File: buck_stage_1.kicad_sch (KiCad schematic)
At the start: 30 parts

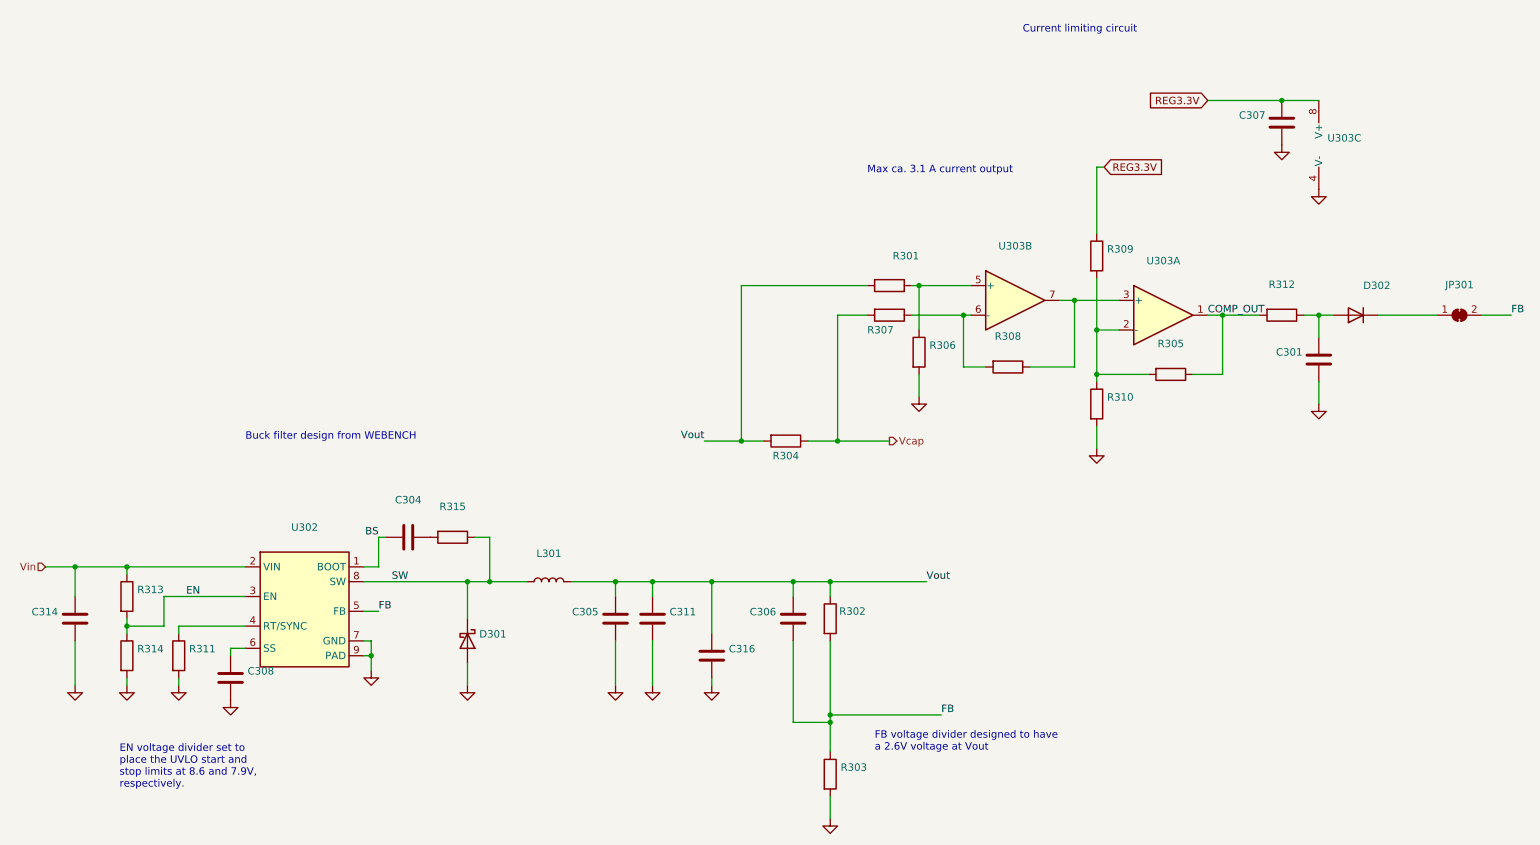
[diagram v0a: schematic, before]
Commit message: SH-RPi v2 schematic design
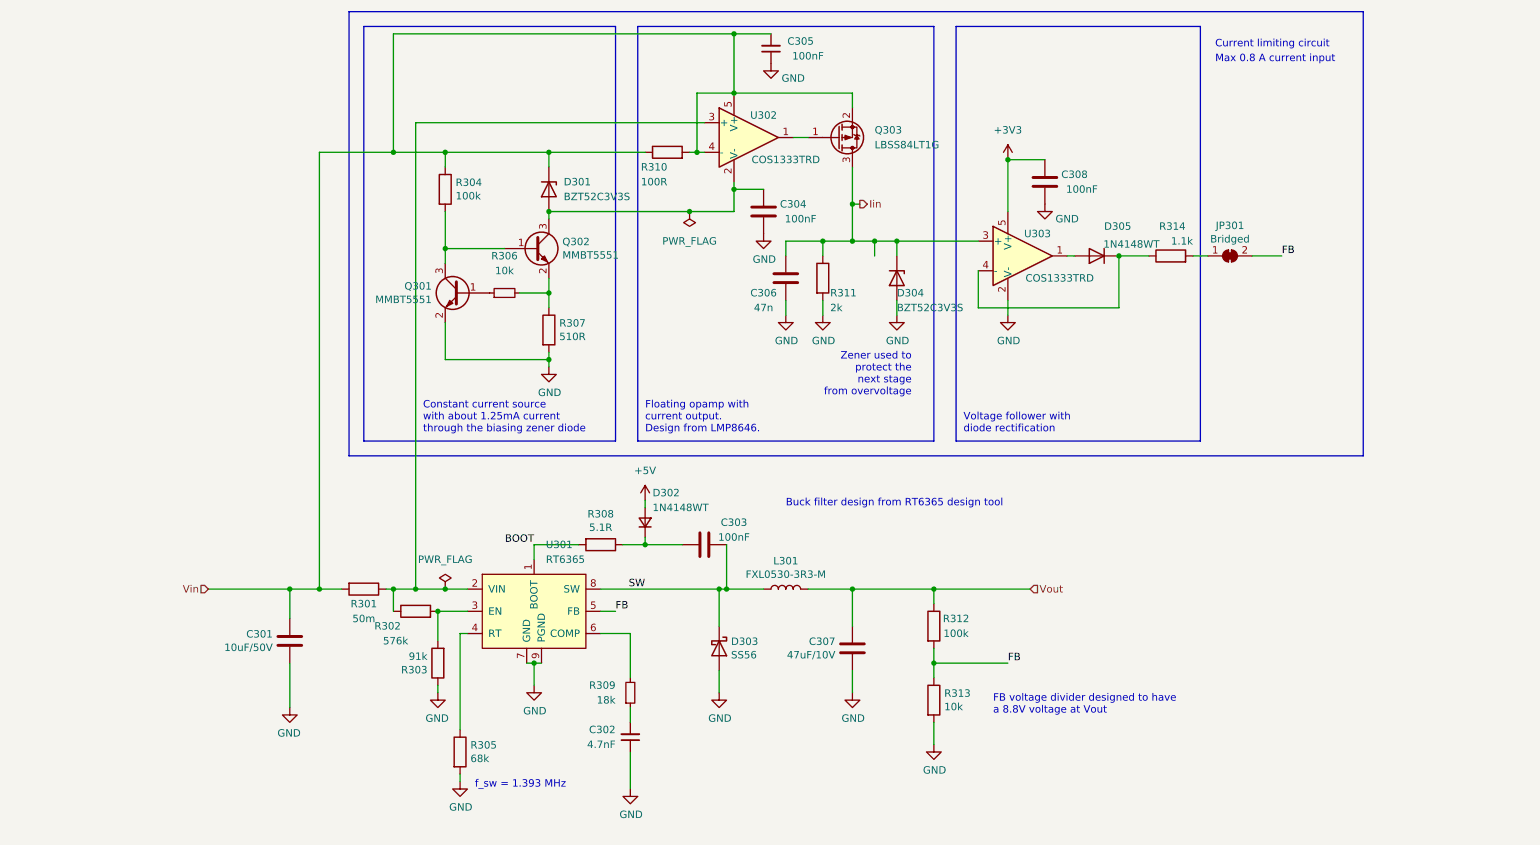
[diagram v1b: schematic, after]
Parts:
- removed C301, C308, C311, C316: (no value), symbol Device:C
- removed R301, R305, R306, R308, R309, R312, R313: (no value), symbol Device:R
- removed U302: (no value), symbol SH-RPi:LMR14050SDDA
- removed U303: (no value), symbol SH-RPi:GS8052
- added C302: 4.7nF, symbol Device:C_Small
- added C304: 100nF, Capacitor_SMD:C_0402_1005Metric, symbol Device:C
- added C305: 100nF, Capacitor_SMD:C_0402_1005Metric, symbol Device:C_Small
- added D301, D304: BZT52C3V3S, Diode_SMD:D_SOD-323, symbol Device:D_Zener
- added D302: 1N4148WT, Diode_SMD:D_SOD-523, symbol Device:D_Small
- added Q301, Q302: MMBT5551, Package_TO_SOT_SMD:SOT-23, symbol Transistor_BJT:MMBT5551L
- added Q303: LBSS84LT1G, Package_TO_SOT_SMD:SOT-23, symbol Transistor_FET:BSS84
- added R302: 576k, Resistor_SMD:R_0402_1005Metric, symbol Device:R
- added R303: 91k, Resistor_SMD:R_0402_1005Metric, symbol Device:R
- added R304: 100k, symbol Device:R
- added R306: 10k, symbol Device:R_Small
- added R309: 18k, symbol Device:R_Small
- added R311: 2k, symbol Device:R
- added U301: RT6365, symbol SH-RPi:RT6365
- added U302, U303: COS1333TRD, Package_TO_SOT_SMD:SOT-23-5, symbol SH-RPi:COS1333
- C301: renamed from C314; value (none) -> 10uF/50V; footprint (none) -> Capacitor_SMD:C_1206_3216Metric; LCSC C13585 -> (none)
- C303: renamed from C304; value (none) -> 100nF; footprint (none) -> Capacitor_SMD:C_0603_1608Metric; LCSC C1525 -> (none)
- C306: value (none) -> 47n; LCSC C15195 -> (none)
- C307: renamed from C305; value (none) -> 47uF/10V; footprint (none) -> Capacitor_SMD:C_0805_2012Metric; LCSC C16780 -> (none); Notes Min 6.3V -> Min 10V
- C308: renamed from C307; value (none) -> 100nF; footprint (none) -> Capacitor_SMD:C_0402_1005Metric
- D303: renamed from D301; value (none) -> SS56; footprint (none) -> Diode_SMD:D_SMA; LCSC C22452 -> C65009
- D305: renamed from D302; value (none) -> 1N4148WT; footprint (none) -> Diode_SMD:D_SOD-523
- JP301: value (none) -> Bridged; footprint (none) -> Jumper:SolderJumper-2_P1.3mm_Bridged_Pad1.0x1.5mm
- L301: value (none) -> FXL0530-3R3-M; footprint (none) -> SH-RPi:L_MWSA0503S; LCSC C285700 -> C475518
- R301: renamed from R304; value (none) -> 50m; footprint (none) -> Resistor_SMD:R_1206_3216Metric; LCSC C127703 -> (none)
- R305: renamed from R311; value (none) -> 68k; footprint (none) -> Resistor_SMD:R_0402_1005Metric; LCSC C25783 -> (none)
- R307: value (none) -> 510R; LCSC C25768 -> (none)
- R308: renamed from R315; value (none) -> 5.1R; footprint (none) -> Resistor_SMD:R_0603_1608Metric
- R310: value (none) -> 100R; LCSC C25918 -> (none)
- R312: renamed from R302; value (none) -> 100k; footprint (none) -> Resistor_SMD:R_0402_1005Metric; LCSC C25774 -> (none)
- R313: renamed from R303; value (none) -> 10k; footprint (none) -> Resistor_SMD:R_0402_1005Metric; LCSC C25750 -> (none)
- R314: value (none) -> 1.1k; LCSC C25769 -> (none)
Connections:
- net EN is gone; now on an unnamed net: R314.1
- net FB: now also U301.5 (FB); no longer C306.2
- net GND: now also C306.1, R307.2, C302.1, C304.1, C305.1, D304.2 (A), Q301.2 (E), R303.1, R311.2, U301.7 (GND), U301.9 (PGND), U303.2 (V-); no longer R310.2, R314.2
- net SW: now also C303.1, U301.8 (SW); no longer R308.1
- net Vin: now also R301.2, R310.1, R310.2, C305.2, D301.1 (K), Q303.2 (S), R304.1, U302.4 (-), U302.5 (V+)
- net Vout: no longer C306.1, R301.2
- net BOOT: now reaches R308.2
- net BOOT: now also U301.1 (BOOT); no longer C303.1
- net at D305.1 (K): now also U303.4 (-); no longer JP301.1 (A)
- net at D305.2 (A): now also U303.1
- net at R307.1: now also Q302.2 (E), R306.2
- net at R305.1: now also U301.4 (RT)
- net BS: no longer names the net of C303.2
- net BS: now also R308.1, D302.1 (K)
- net REG3.3V renamed +3V3
- net +3V3: now also U303.5 (V+)
- net Vcap: no longer names the net of R301.1
- net Vcap: now also R302.1, U301.2 (VIN), U302.3 (+); no longer R307.2
- new net: JP301.1 (A), R314.2
- new net: R302.2, R303.2, U301.3 (EN)
- new net: R309.2, U301.6 (COMP)
- new net: Q303.1 (G), U302.1
- new net: C304.2, D301.2 (A), Q302.3 (C), U302.2 (V-)
- new net: Q301.3 (C), Q302.1 (B), R304.2
- new net: C302.2, R309.1
- new net: Q301.1 (B), R306.1
- new net +5V: D302.2 (A)
- new net Iin: C306.2, D304.1 (K), Q303.3 (D), R311.1, U303.3 (+)
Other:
- note added: "Buck filter design from RT6365 design tool"
- note added: "Constant current source with about 1.25mA current through the biasing zener diode"
- note added: "FB voltage divider designed to have a 8.8V voltage at Vout"
- note added: "Floating opamp with current output. Design from LMP8646."
- note added: "Max 0.8 A current input"
- note added: "Voltage follower with diode rectification"
- note added: "Zener used to protect the next stage from overvoltage"
- note added: "f_sw = 1.393 MHz"
- note removed: "Buck filter design from WEBENCH"
- note removed: "EN voltage divider set to place the UVLO start and stop limits at 8.6 and 7.9V, respectively."
- note removed: "FB voltage divider designed to have a 2.6V voltage at Vout"
- note removed: "Max ca. 3.1 A current output"
- moved on the sheet: C301, C303, C307, C308, D303, D305, JP301, L301, R301, R305, R308, R312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
